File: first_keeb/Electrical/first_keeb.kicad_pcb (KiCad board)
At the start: 2 copper layers, 97.2 x 65.2 mm, 20 parts, among them U1 RPi_Pico_SMD_TH

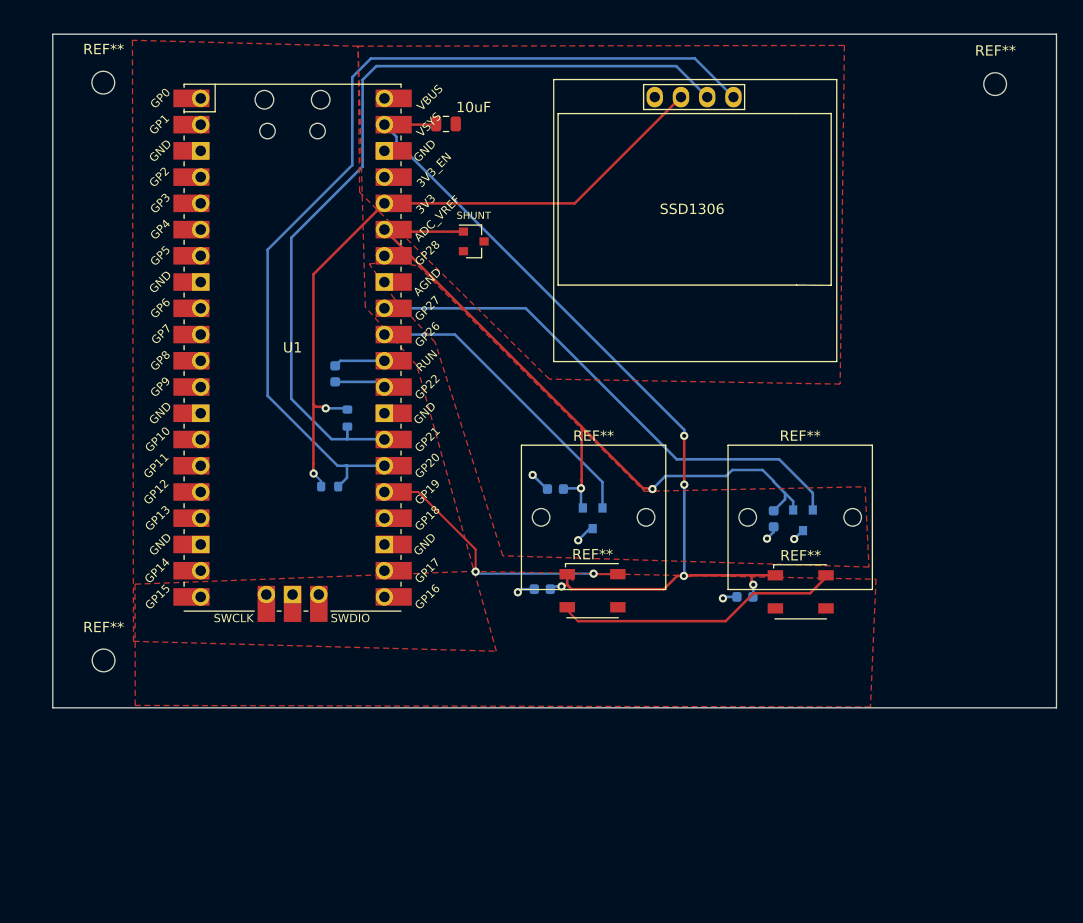
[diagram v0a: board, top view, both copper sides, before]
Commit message: improve pcb
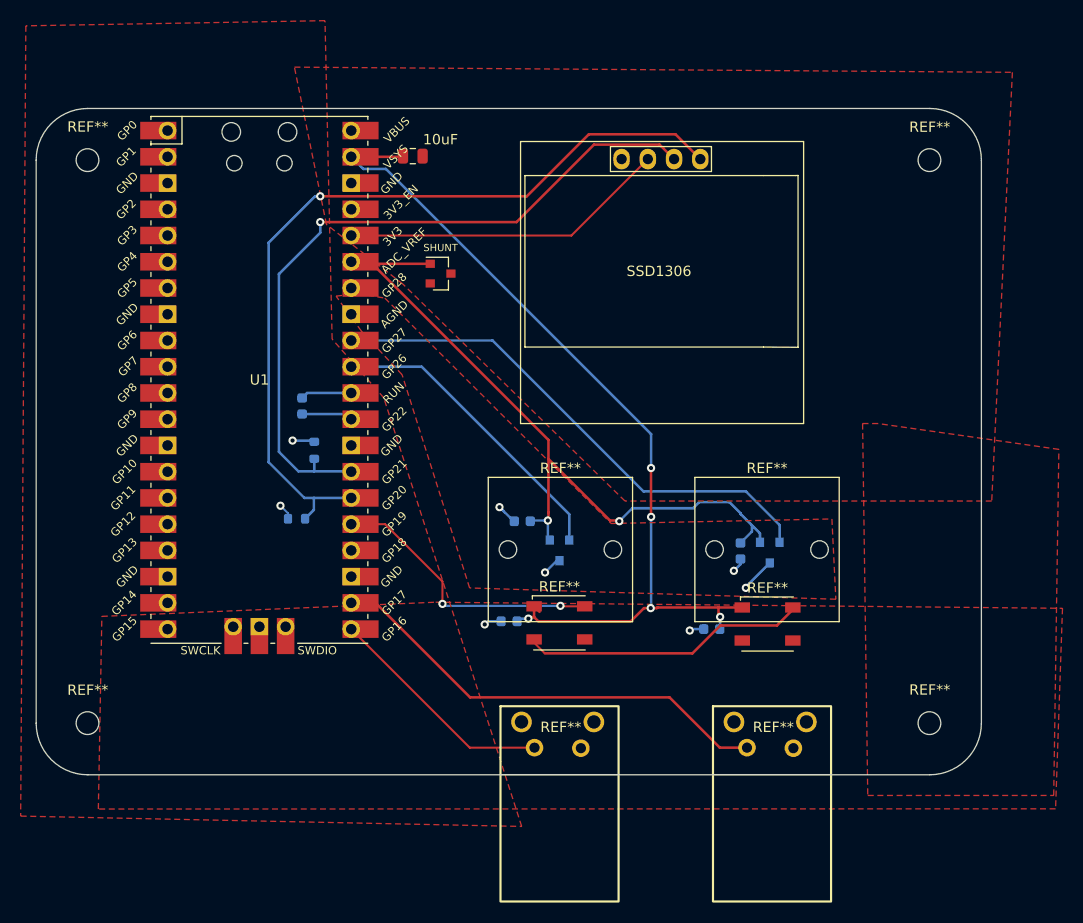
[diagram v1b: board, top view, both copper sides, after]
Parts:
- added REF**: MountingHole_2.2mm_M2, MountingHole:MountingHole_2.2mm_M2, F.Cu at (105.0, 125.0)
- added REF**: 2-1825027-0_Right_Angle_Switch-9.24mm_Stem, Button_Switch_THT:2-1825027-0_Right_Angle_Button, F.Cu at (86.0, 124.9)
- added REF**: 2-1825027-0_Right_Angle_Switch-9.24mm_Stem, Button_Switch_THT:2-1825027-0_Right_Angle_Button, F.Cu at (65.5, 124.9)
- moved REF** 9.74 mm to (105.0, 70.5)
- moved REF** 7.65 mm to (23.5, 70.5)
- moved SSD1306 6.80 mm to (78.8, 81.0)
- moved REF** 6.26 mm to (23.5, 125.0)
- moved PULL 4.47 mm to (43.7, 105.2)
- moved RST 4.47 mm to (44.2, 94.3)
- moved CUP 4.47 mm to (64.3, 115.1)
- moved REF** 4.47 mm to (89.5, 108.5)
- moved REF** 4.47 mm to (89.3, 115.4)
- moved SENS 4.47 mm to (69.2, 108.3)
- moved 10uF 4.47 mm to (55.0, 70.1)
- moved PULL 4.47 mm to (45.4, 98.6)
- moved SHUNT 4.47 mm to (57.6, 81.5)
- moved U1 4.47 mm to (40.1, 91.8)
- moved CUP 4.47 mm to (83.9, 115.9)
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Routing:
- net (no net): track 545.3 -> 559.3 mm
- net GND: track 3.13 -> 7.09 mm, vias 2 -> 4
- net AGND: track 5.52 -> 7.71 mm
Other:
- board size 97.2 x 65.2 mm -> 91.5 x 64.5 mm
